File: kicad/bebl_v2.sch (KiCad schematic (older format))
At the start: 78 parts, among them P1 ISP, P10 LED_DRL, P11 DRV_LED, P12 CHG_LED, P13 LED_CHG, P2 FTDI, P3 LiPo, P4 USB-Micro, P5 Alt_Add, P6 Int1, P7 Int2, P8 DRL_LED, P9 LED_DRV, SW1 RST, SW2 MODE, U1 ATMEGA328, U2 FAN5346, U3 ADXL345, U4 MCP73831, U5 TPS61221DCK, X1 8MHz

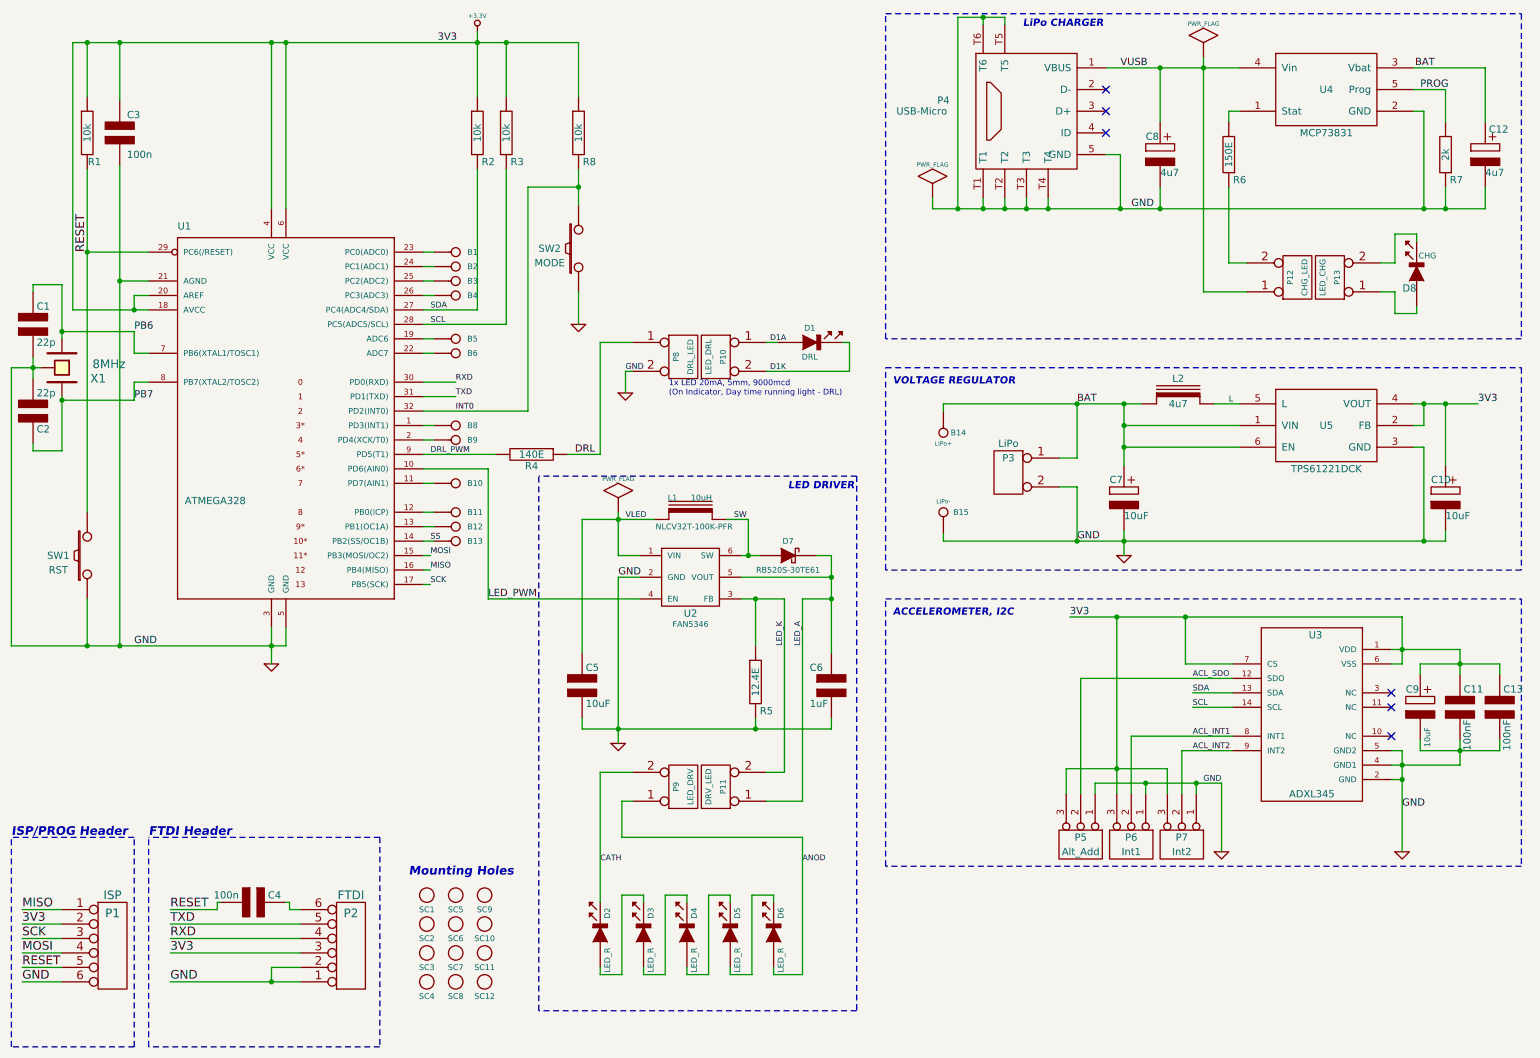
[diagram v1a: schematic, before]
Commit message: working on case for bebl_v2
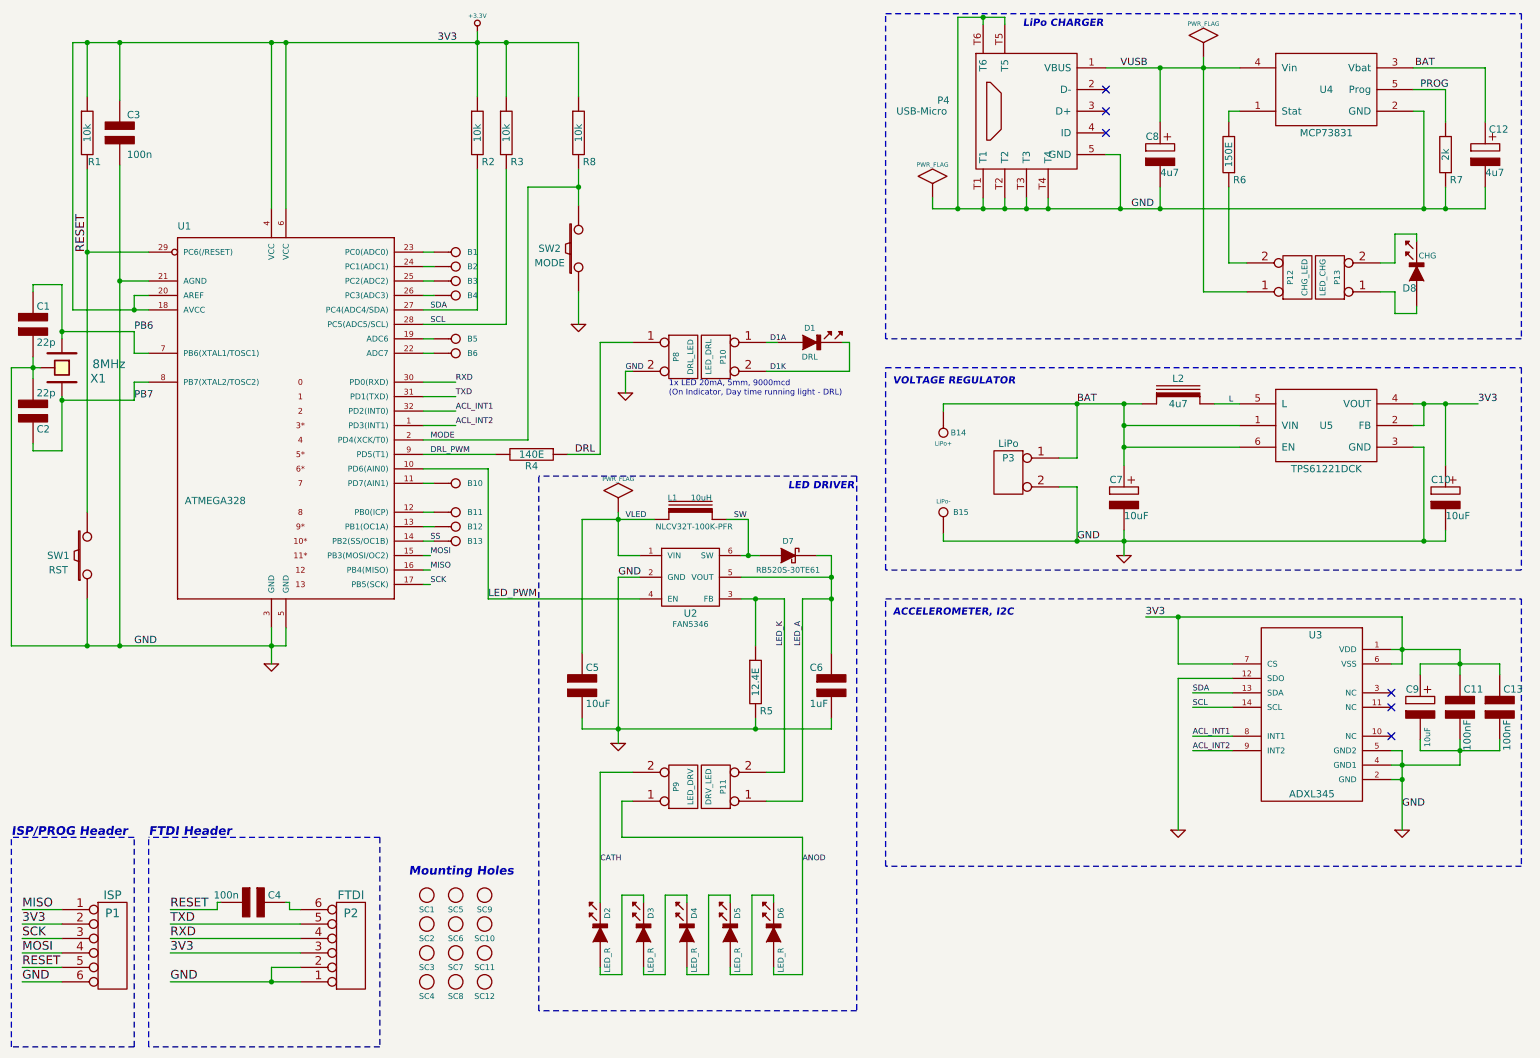
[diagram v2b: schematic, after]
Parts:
- removed B8, B9: I/O, bebl_v2_pretty:breakout_smd, symbol I/O
- removed P5: Alt_Add, bebl_v2_pretty:solder_bridge_3, symbol CONN_3
- removed P6: Int1, bebl_v2_pretty:solder_bridge_3, symbol CONN_3
- removed P7: Int2, bebl_v2_pretty:solder_bridge_3, symbol CONN_3
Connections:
- net ACL_SDO is gone; now on net GND: U3.12 (SDO)
- net ACL_INT1: now also U1.32 (PD2(INT0))
- net ACL_INT2: now also U1.1 (PD3(INT1))
- net MODE: now reaches U1.2 (PD4(XCK/T0))
- net MODE: now also R8.2, SW2.2
- removed net INT0: R8.2, SW2.2, U1.32 (PD2(INT0))
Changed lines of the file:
@@
 NoConn ~ 10100 5400
 Wire Wire Line
-	10175 5700 10175 6400
+	10175 5700 10175 6250
 Wire Wire Line
 	10100 5900 10175 5900
@@
 L GND #PWR04
 U 1 1 542E7DB5
-P 10175 6400
-F 0 "#PWR04" H 10175 6400 30  0001 C CNN
-F 1 "GND" H 10175 6330 30  0001 C CNN
-F 2 "" H 10175 6400 60  0001 C CNN
-F 3 "" H 10175 6400 60  0001 C CNN
-	1    10175 6400
+P 10175 6250
+F 0 "#PWR04" H 10175 6250 30  0001 C CNN
+F 1 "GND" H 10175 6180 30  0001 C CNN
+F 2 "" H 10175 6250 60  0001 C CNN
+F 3 "" H 10175 6250 60  0001 C CNN
+	1    10175 6250
 	1    0    0    -1
 $EndComp
@@
 	10575 5000 10575 5175
 Connection ~ 10575 5100
-Text Label 8725 5200 0    40   ~ 0
-ACL_SDO
-Wire Wire Line
-	8300 5600 9000 5600
-Wire Wire Line
-	8650 5700 9000 5700
+Wire Wire Line
+	8725 5600 9000 5600
+Wire Wire Line
+	8725 5700 9000 5700
 Wire Wire Line
 	9000 5400 8725 5400
@@
 	8725 5300 9000 5300
 Wire Wire Line
-	7950 5200 9000 5200
-Wire Wire Line
-	8675 5100 9000 5100
+	8625 5200 9000 5200
+Wire Wire Line
+	8625 5100 9000 5100
 Text Label 8725 5400 0    40   ~ 0
 SCL
@@
 ACL_INT2
 Wire Wire Line
-	7875 4775 10175 4775
-Wire Wire Line
-	8675 5100 8675 4775
-Connection ~ 8675 4775
-$Comp
-L CONN_3 P5
-U 1 1 542E7E0B
-P 7950 6350
-F 0 "P5" V 7900 6350 50  0000 C CNN
-F 1 "Alt_Add" V 8000 6350 50  0000 C CNN
-F 2 "bebl_v2_pretty:solder_bridge_3" H 7950 6350 60  0001 C CNN
-F 3 "" H 7950 6350 60  0000 C CNN
-F 4 "CONN HEADER 50POS .100\" SGL GOLD" H 7950 6450 60  0001 L CNN "Field4"
-F 5 "Header, Unshrouded, Male pin," H 7950 6550 60  0001 L CNN "Field5"
-F 6 "0.1\" pitch x 50 nos" H 7950 6650 60  0001 L CNN "Field6"
-F 7 "Samtec Inc" H 7950 6750 60  0001 L CNN "Field7"
-F 8 "TSW-150-07-L-S" H 7950 6850 60  0001 L CNN "Field8"
-F 9 "Digikey" H 7950 6950 60  0001 L CNN "Field9"
-F 10 "SAM1031-50-ND" H 7950 7050 60  0001 L CNN "Field10"
-F 11 "http://www.digikey.com/scripts/DkSearch/dksus.dll?WT.z_header=search_go&lang=en&keywords=SAM1031-50-ND&x=15&y=16&cur=USD" H 7950 7150 60  0001 L CNN "Field11"
-	1    7950 6350
-	0    1    1    0
-$EndComp
-$Comp
-L CONN_3 P6
-U 1 1 542E7E19
-P 8300 6350
-F 0 "P6" V 8250 6350 50  0000 C CNN
-F 1 "Int1" V 8350 6350 50  0000 C CNN
-F 2 "bebl_v2_pretty:solder_bridge_3" H 8300 6350 60  0001 C CNN
-F 3 "" H 8300 6350 60  0000 C CNN
-F 4 "CONN HEADER 50POS .100\" SGL GOLD" H 8300 6450 60  0001 L CNN "Field4"
-F 5 "Header, Unshrouded, Male pin," H 8300 6550 60  0001 L CNN "Field5"
-F 6 "0.1\" pitch x 50 nos" H 8300 6650 60  0001 L CNN "Field6"
-F 7 "Samtec Inc" H 8300 6750 60  0001 L CNN "Field7"
-F 8 "TSW-150-07-L-S" H 8300 6850 60  0001 L CNN "Field8"
-F 9 "Digikey" H 8300 6950 60  0001 L CNN "Field9"
-F 10 "SAM1031-50-ND" H 8300 7050 60  0001 L CNN "Field10"
-F 11 "http://www.digikey.com/scripts/DkSearch/dksus.dll?WT.z_header=search_go&lang=en&keywords=SAM1031-50-ND&x=15&y=16&cur=USD" H 8300 7150 60  0001 L CNN "Field11"
-	1    8300 6350
-	0    1    1    0
-$EndComp
-$Comp
-L CONN_3 P7
-U 1 1 542E7E27
-P 8650 6350
-F 0 "P7" V 8600 6350 50  0000 C CNN
-F 1 "Int2" V 8700 6350 50  0000 C CNN
-F 2 "bebl_v2_pretty:solder_bridge_3" H 8650 6350 60  0001 C CNN
-F 3 "" H 8650 6350 60  0000 C CNN
-F 4 "CONN HEADER 50POS .100\" SGL GOLD" H 8650 6450 60  0001 L CNN "Field4"
-F 5 "Header, Unshrouded, Male pin," H 8650 6550 60  0001 L CNN "Field5"
-F 6 "0.1\" pitch x 50 nos" H 8650 6650 60  0001 L CNN "Field6"
-F 7 "Samtec Inc" H 8650 6750 60  0001 L CNN "Field7"
-F 8 "TSW-150-07-L-S" H 8650 6850 60  0001 L CNN "Field8"
-F 9 "Digikey" H 8650 6950 60  0001 L CNN "Field9"
-F 10 "SAM1031-50-ND" H 8650 7050 60  0001 L CNN "Field10"
-F 11 "http://www.digikey.com/scripts/DkSearch/dksus.dll?WT.z_header=search_go&lang=en&keywords=SAM1031-50-ND&x=15&y=16&cur=USD" H 8650 7150 60  0001 L CNN "Field11"
-	1    8650 6350
-	0    1    1    0
-$EndComp
-Wire Wire Line
-	8650 6000 8650 5700
-Wire Wire Line
-	8300 5600 8300 6000
-Wire Wire Line
-	7950 6000 7950 5200
-Wire Wire Line
-	8550 5825 8550 6000
-Wire Wire Line
-	7850 5825 8550 5825
-Wire Wire Line
-	7850 5825 7850 6000
-Wire Wire Line
-	8200 4775 8200 6000
-Connection ~ 8200 5825
-Connection ~ 8200 4775
-Wire Wire Line
-	8050 6000 8050 5925
-Wire Wire Line
-	8050 5925 8925 5925
-Wire Wire Line
-	8750 5925 8750 6000
-Wire Wire Line
-	8400 6000 8400 5925
-Connection ~ 8400 5925
-Wire Wire Line
-	8925 5925 8925 6400
-Connection ~ 8750 5925
+	8400 4775 10175 4775
+Wire Wire Line
+	8625 5100 8625 4775
+Connection ~ 8625 4775
+Wire Wire Line
+	8625 6250 8625 5200
 $Comp
 L GND #PWR05
 U 1 1 542E7E3D
-P 8925 6400
-F 0 "#PWR05" H 8925 6400 30  0001 C CNN
-F 1 "GND" H 8925 6330 30  0001 C CNN
-F 2 "" H 8925 6400 60  0001 C CNN
-F 3 "" H 8925 6400 60  0001 C CNN
-	1    8925 6400
-	1    0    0    -1
-$EndComp
-Text Label 8925 5925 2    40   ~ 0
-GND
+P 8625 6250
+F 0 "#PWR05" H 8625 6250 30  0001 C CNN
+F 1 "GND" H 8625 6180 30  0001 C CNN
+F 2 "" H 8625 6250 60  0001 C CNN
+F 3 "" H 8625 6250 60  0001 C CNN
+	1    8625 6250
+	1    0    0    -1
+$EndComp
 Text Label 10175 6100 0    50   ~ 0
 GND
 Text Label 8725 5300 0    40   ~ 0
 SDA
-Text Label 7875 4775 0    50   ~ 0
+Text Label 8400 4775 0    50   ~ 0
 3V3
 $Comp
@@
 $EndComp
 $Comp
-L I/O B8
-U 1 1 54312216
-P 3625 3450
-F 0 "B8" H 3705 3450 40  0000 L CNN
-F 1 "I/O" H 3625 3505 30  0001 C CNN
-F 2 "bebl_v2_pretty:breakout_smd" H 3625 3450 60  0001 C CNN
-F 3 "" H 3625 3450 60  0000 C CNN
-	1    3625 3450
-	1    0    0    -1
-$EndComp
-$Comp
-L I/O B9
-U 1 1 5431222A
-P 3625 3550
-F 0 "B9" H 3705 3550 40  0000 L CNN
-F 1 "I/O" H 3625 3605 30  0001 C CNN
-F 2 "bebl_v2_pretty:breakout_smd" H 3625 3550 60  0001 C CNN
-F 3 "" H 3625 3550 60  0000 C CNN
-	1    3625 3550
-	1    0    0    -1
-$EndComp
-$Comp
 L I/O B10
 U 1 1 5431223E
@@
 Wire Wire Line
 	3475 4050 3400 4050
-Wire Wire Line
-	3400 3550 3475 3550
 Wire Wire Line
 	3400 3850 3475 3850
@@
 Text Notes 7550 700  0    50   Italic 10
 LiPo CHARGER
-Wire Wire Line
-	3400 3350 4125 3350
 Text Label 10300 1125 0    50   ~ 0
 PROG
@@
 Wire Wire Line
 	3400 3750 3850 3750
-Wire Wire Line
-	3475 3450 3400 3450
 Wire Wire Line
 	3400 3650 3900 3650
@@
 $EndComp
 Wire Wire Line
-	4125 3350 4125 1800
+	4125 1800 4125 3550
 Wire Wire Line
 	4125 1800 4475 1800
@@
 	1    0    0    -1
 $EndComp
-Text Label 3625 3350 0    40   ~ 0
-INT0
 Wire Wire Line
 	4625 3650 4625 2875
@@
 Wire Wire Line
 	8975 2325 9100 2325
+Wire Wire Line
+	4125 3550 3400 3550
+Wire Wire Line
+	3400 3350 3625 3350
+Wire Wire Line
+	3400 3450 3625 3450
+Text Label 3450 3550 0    40   ~ 0
+MODE
+Text Label 3625 3350 0    40   ~ 0
+ACL_INT1
+Text Label 3625 3450 0    40   ~ 0
+ACL_INT2
 $EndSCHEMATC
